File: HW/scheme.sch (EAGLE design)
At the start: 7 parts, among them IC1 FT245RL

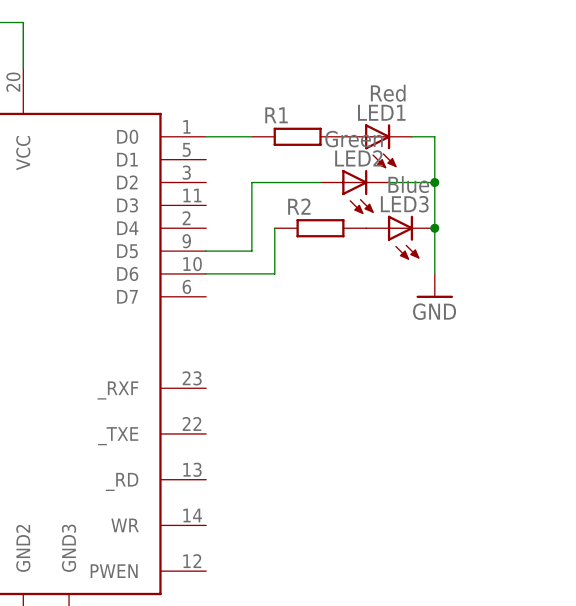
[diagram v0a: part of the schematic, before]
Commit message: Board v2
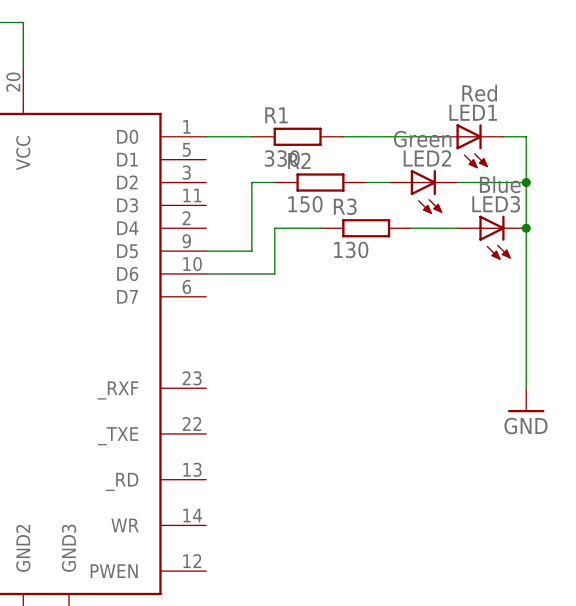
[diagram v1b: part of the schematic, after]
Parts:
- added R3: 130, resistor:R-EU_M1406
- LED1, LED2: device led:LED5MM -> led:NFSG036BT
- LED3: device led:LED3MM -> led:NFSG036BT
- R1: value (none) -> 330; device resistor:R-EU_0204/5 -> resistor:R-EU_M1406
- R2: value (none) -> 150; device resistor:R-EU_0204/5 -> resistor:R-EU_M1406
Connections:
- new net N$9: LED3.A, R3.2
- net N$5: now also R3.1; no longer R2.1
- net N$6: now also R2.1; no longer LED2.A
- net N$7: now also LED2.A; no longer LED3.A
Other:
- moved on the sheet: LED1, LED2, LED3, R2
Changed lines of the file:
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@@
 <part name="GND1" library="supply1" deviceset="GND" device=""/>
 <part name="GND2" library="supply1" deviceset="GND" device=""/>
-<part name="LED1" library="led" deviceset="LED" device="5MM" value="Red"/>
-<part name="LED2" library="led" deviceset="LED" device="5MM" value="Green"/>
-<part name="LED3" library="led" deviceset="LED" device="3MM" value="Blue"/>
+<part name="LED1" library="led" deviceset="NFSG036BT" device="" value="Red"/>
+<part name="LED2" library="led" deviceset="NFSG036BT" device="" value="Green"/>
+<part name="LED3" library="led" deviceset="NFSG036BT" device="" value="Blue"/>
 <part name="GND3" library="supply1" deviceset="GND" device=""/>
-<part name="R1" library="resistor" deviceset="R-EU_" device="0204/5"/>
-<part name="R2" library="resistor" deviceset="R-EU_" device="0204/5"/>
+<part name="R1" library="resistor" deviceset="R-EU_" device="M1406" value="330"/>
 <part name="X1" library="shmuma" deviceset="USB-A003" device="BOTTOM"/>
+<part name="R3" library="resistor" deviceset="R-EU_" device="M1406" value="130"/>
+<part name="R2" library="resistor" deviceset="R-EU_" device="M1406" value="150"/>
 </parts>
 <sheets>
@@
 <instance part="GND1" gate="1" x="17.78" y="15.24"/>
 <instance part="GND2" gate="1" x="-20.32" y="83.82" rot="R180"/>
-<instance part="LED1" gate="G$1" x="66.04" y="76.2" rot="R90"/>
-<instance part="LED2" gate="G$1" x="63.5" y="71.12" rot="R90"/>
-<instance part="LED3" gate="G$1" x="68.58" y="66.04" rot="R90"/>
-<instance part="GND3" gate="1" x="73.66" y="58.42"/>
+<instance part="LED1" gate="G$1" x="76.2" y="76.2" rot="R90"/>
+<instance part="LED2" gate="G$1" x="71.12" y="71.12" rot="R90"/>
+<instance part="LED3" gate="G$1" x="78.74" y="66.04" rot="R90"/>
+<instance part="GND3" gate="1" x="83.82" y="45.72"/>
 <instance part="R1" gate="G$1" x="58.42" y="76.2"/>
-<instance part="R2" gate="G$1" x="60.96" y="66.04"/>
 <instance part="X1" gate="G$1" x="-27.94" y="73.66" rot="R180"/>
+<instance part="R3" gate="G$1" x="66.04" y="66.04"/>
+<instance part="R2" gate="G$1" x="60.96" y="71.12"/>
 </instances>
 <busses>
@@
 <pinref part="LED1" gate="G$1" pin="C"/>
 <pinref part="GND3" gate="1" pin="GND"/>
-<wire x1="71.12" y1="76.2" x2="73.66" y2="76.2" width="0.1524" layer="91"/>
-<wire x1="73.66" y1="76.2" x2="73.66" y2="71.12" width="0.1524" layer="91"/>
+<wire x1="81.28" y1="76.2" x2="83.82" y2="76.2" width="0.1524" layer="91"/>
+<wire x1="83.82" y1="76.2" x2="83.82" y2="71.12" width="0.1524" layer="91"/>
 <pinref part="LED3" gate="G$1" pin="C"/>
-<wire x1="73.66" y1="71.12" x2="73.66" y2="66.04" width="0.1524" layer="91"/>
-<wire x1="73.66" y1="66.04" x2="73.66" y2="60.96" width="0.1524" layer="91"/>
+<wire x1="83.82" y1="71.12" x2="83.82" y2="66.04" width="0.1524" layer="91"/>
 <pinref part="LED2" gate="G$1" pin="C"/>
-<wire x1="68.58" y1="71.12" x2="73.66" y2="71.12" width="0.1524" layer="91"/>
-<junction x="73.66" y="66.04"/>
-<junction x="73.66" y="71.12"/>
+<wire x1="83.82" y1="66.04" x2="83.82" y2="48.26" width="0.1524" layer="91"/>
+<wire x1="76.2" y1="71.12" x2="83.82" y2="71.12" width="0.1524" layer="91"/>
+<junction x="83.82" y="66.04"/>
+<junction x="83.82" y="71.12"/>
 </segment>
 <segment>
@@
 </segment>
 </net>
-<net name="N$7" class="0">
-<segment>
-<pinref part="R2" gate="G$1" pin="2"/>
-<pinref part="LED3" gate="G$1" pin="A"/>
-</segment>
-</net>
 <net name="N$8" class="0">
 <segment>
 <pinref part="R1" gate="G$1" pin="2"/>
 <pinref part="LED1" gate="G$1" pin="A"/>
+<wire x1="73.66" y1="76.2" x2="63.5" y2="76.2" width="0.1524" layer="91"/>
 </segment>
 </net>
@@
 <net name="N$5" class="0">
 <segment>
-<pinref part="R2" gate="G$1" pin="1"/>
-<wire x1="55.88" y1="66.04" x2="55.88" y2="60.96" width="0.1524" layer="91"/>
 <pinref part="IC1" gate="G$1" pin="D6"/>
 <wire x1="55.88" y1="60.96" x2="48.26" y2="60.96" width="0.1524" layer="91"/>
+<wire x1="55.88" y1="60.96" x2="55.88" y2="66.04" width="0.1524" layer="91"/>
+<pinref part="R3" gate="G$1" pin="1"/>
+<wire x1="55.88" y1="66.04" x2="60.96" y2="66.04" width="0.1524" layer="91"/>
 </segment>
 </net>
 <net name="N$6" class="0">
 <segment>
-<pinref part="LED2" gate="G$1" pin="A"/>
-<wire x1="60.96" y1="71.12" x2="53.34" y2="71.12" width="0.1524" layer="91"/>
 <wire x1="53.34" y1="71.12" x2="53.34" y2="63.5" width="0.1524" layer="91"/>
 <pinref part="IC1" gate="G$1" pin="D5"/>
 <wire x1="53.34" y1="63.5" x2="48.26" y2="63.5" width="0.1524" layer="91"/>
+<pinref part="R2" gate="G$1" pin="1"/>
+<wire x1="53.34" y1="71.12" x2="55.88" y2="71.12" width="0.1524" layer="91"/>
 </segment>
 </net>
+<net name="N$7" class="0">
+<segment>
+<pinref part="R2" gate="G$1" pin="2"/>
+<pinref part="LED2" gate="G$1" pin="A"/>
+<wire x1="66.04" y1="71.12" x2="68.58" y2="71.12" width="0.1524" layer="91"/>
+</segment>
+</net>
+<net name="N$9" class="0">
+<segment>
+<pinref part="R3" gate="G$1" pin="2"/>
+<pinref part="LED3" gate="G$1" pin="A"/>
+<wire x1="71.12" y1="66.04" x2="76.2" y2="66.04" width="0.1524" layer="91"/>
+</segment>
+</net>
